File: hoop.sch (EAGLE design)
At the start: 33 parts, among them U1 PIC32MM0064GPL020-I/ML, U2 SGM2200

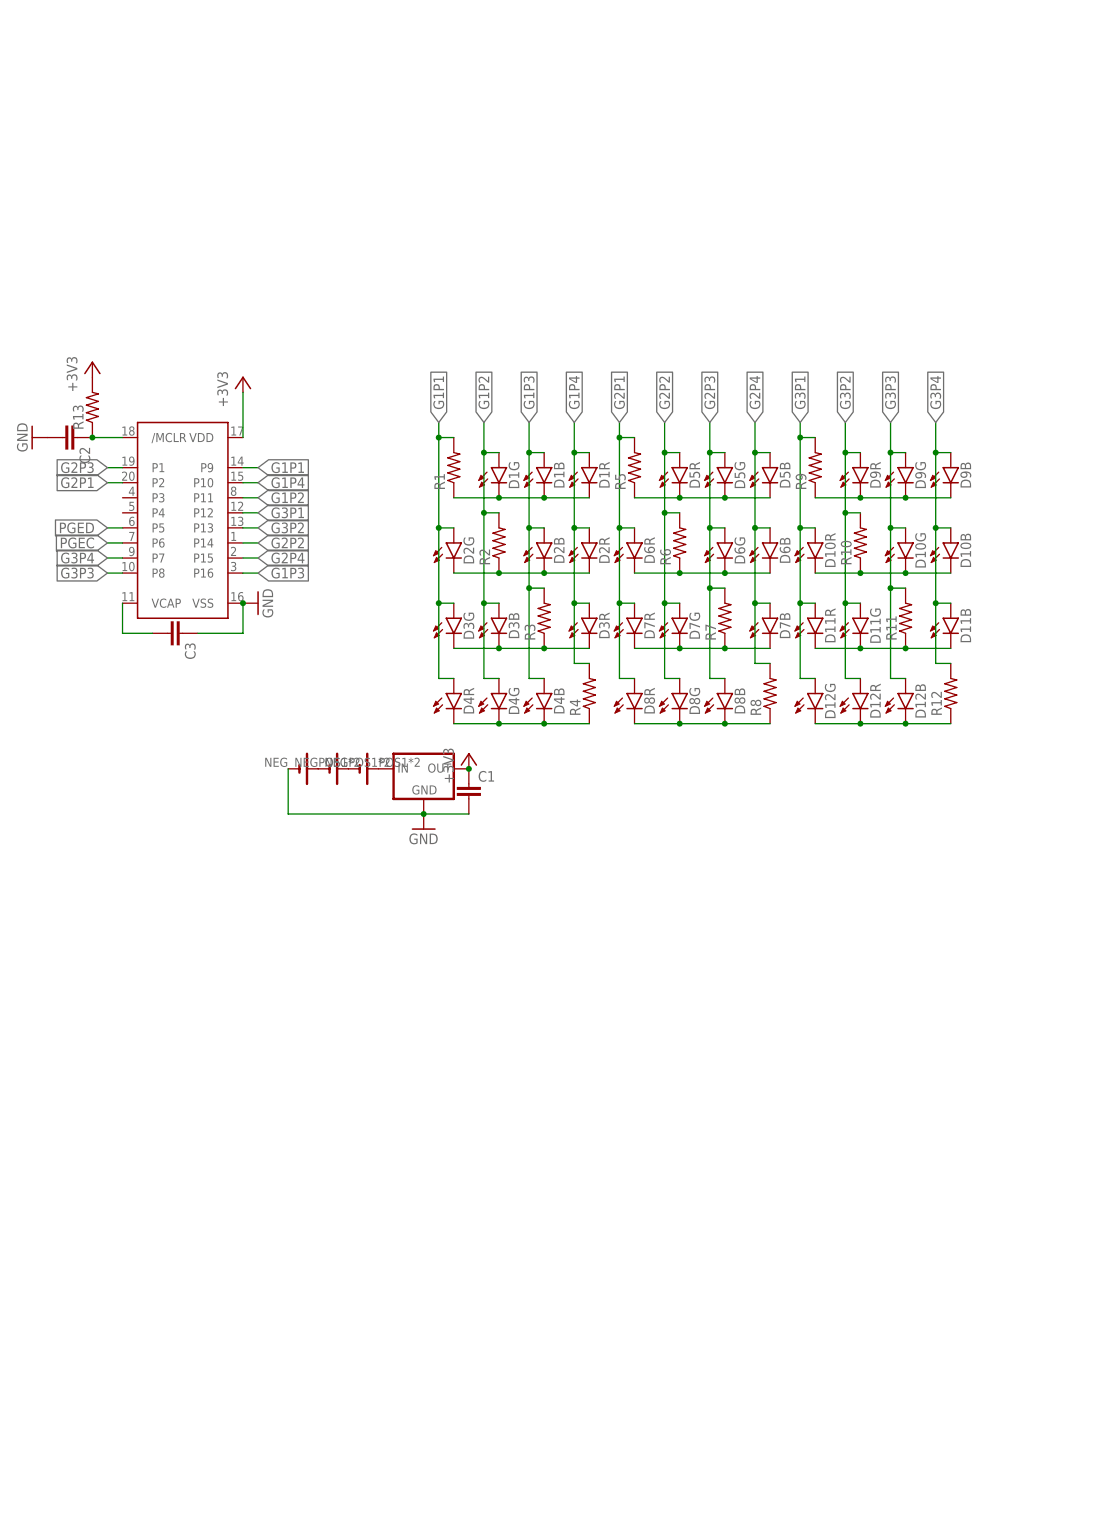
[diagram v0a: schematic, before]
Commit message: Cleaning up pcb files
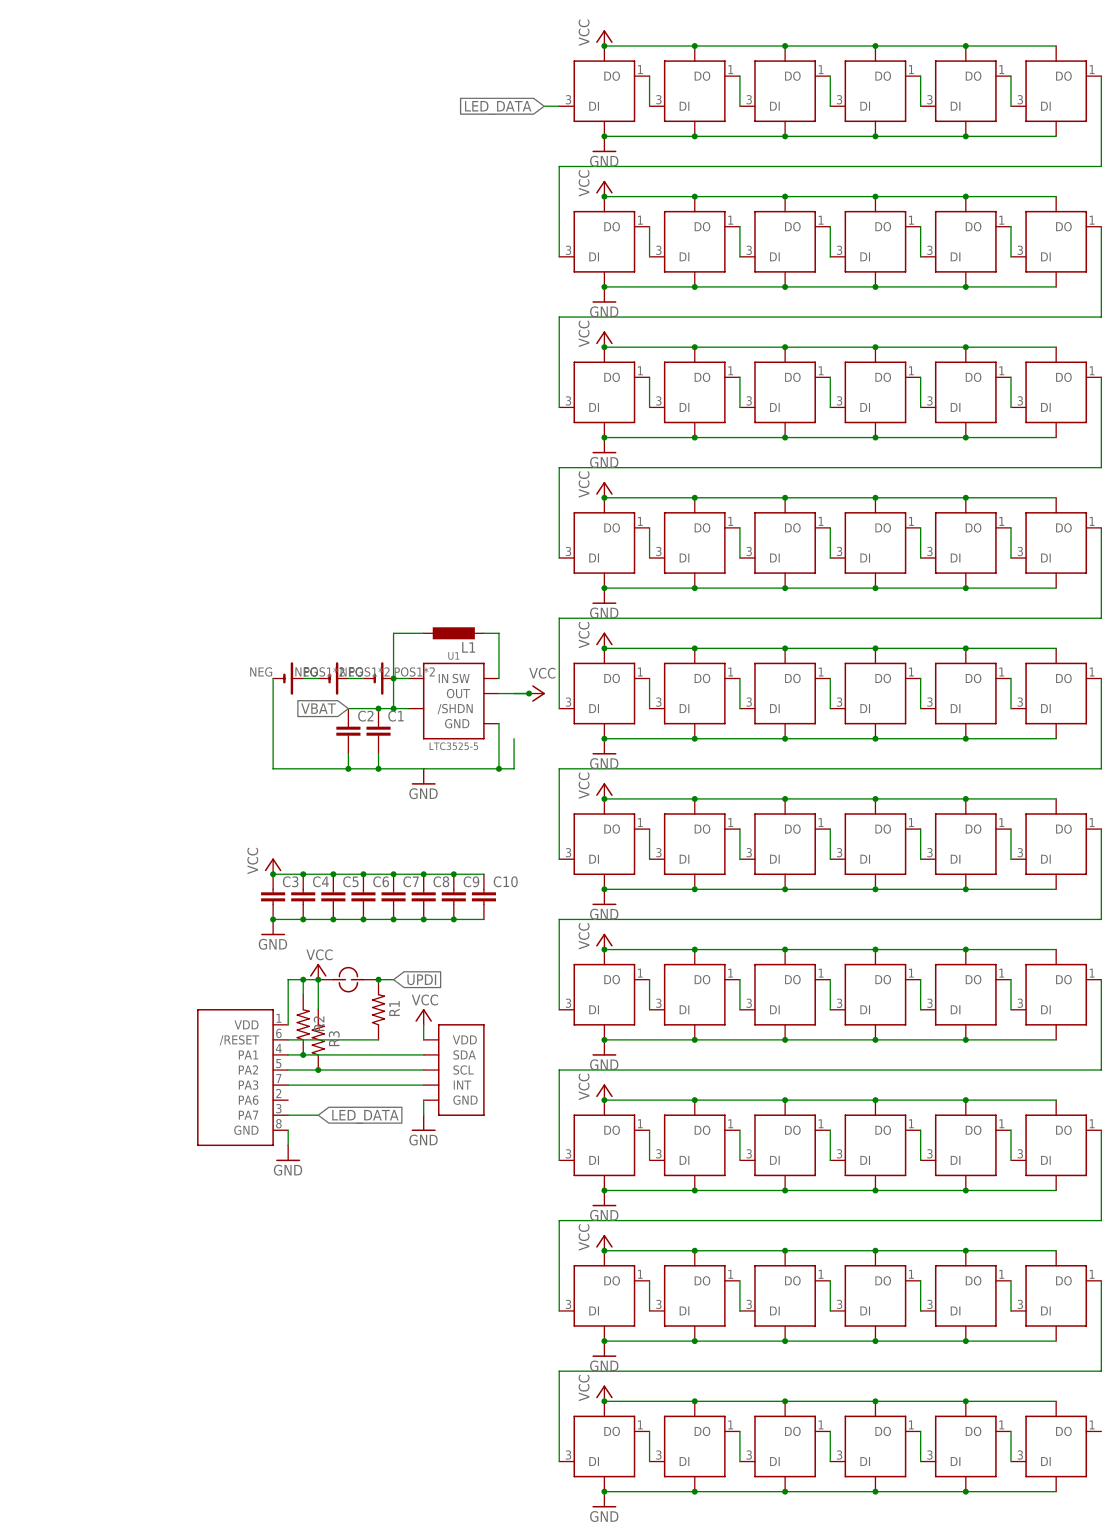
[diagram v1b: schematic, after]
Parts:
- removed R10, R11, R12, R4, R5, R6, R7, R8, R9: (no value), rcl:R-US_R0805
- removed R13: (no value), rcl:R-US_R0402
- added C10, C4, C5, C6, C7, C8, C9: (no value), rcl:C-EUC0805
- added D13, D14, D15, D16, D17, D18, D19, D20, D21, D22, D23, D24, D25, D26, D27, D28, D29, D30, D31, D32, D33, D34, D35, D36, D37, D38, D39, D40, D41, D42, D43, D44, D45, D46, D47, D48, D49, D50, D51, D52, D53, D54, D55, D56, D57, D58, D59, D60: SMD-LX0707RGB-TR, earring:SMD-LX0707RGB-TR
- added J1: JMP, earring:JMP
- added L1: (no value), rcl:L-EUL3216C
- added U3: ATTINY202, earring:ATTINY202
- C1, C2, C3: device rcl:C-EUC0402 -> rcl:C-EUC0805
- D1, D10, D11, D12, D2, D3, D4, D5, D6, D7, D8, D9: value FM-Z2727RGBA-SH -> SMD-LX0707RGB-TR; device earring:FM-Z2727RGBA-SH -> earring:SMD-LX0707RGB-TR
- U1: value PIC32MM0064GPL020-I/ML -> LTC3525; device earring:PIC32MM0064GPL020-I/ML -> earring:LTC3525
- U2: value SGM2200 -> MXC6255XU; device earring:SGM2200 -> earring:MXC6255XU
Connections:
- removed net +3V3: C1.1, R13.2, U1.VDD, U2.OUT
- removed net /MCLR: C2.1, R13.1, U1./MCLR
- removed net G1P1: D2G.A, D3G.A, D4R.A, R1.2, U1.P9
- removed net G1P2: D1G.A, D3B.A, D4G.A, R2.2, U1.P11
- removed net G1P3: D1B.A, D2B.A, D4B.A, R3.2, U1.P16
- removed net G1P4: D1R.A, D2R.A, D3R.A, R4.2, U1.P10
- removed net G2P1: D6R.A, D7R.A, D8R.A, R5.2, U1.P2
- removed net G2P2: D5R.A, D7G.A, D8G.A, R6.2, U1.P14
- removed net G2P3: D5G.A, D6G.A, D8B.A, R7.2, U1.P1
- removed net G2P4: D5B.A, D6B.A, D7B.A, R8.2, U1.P15
- removed net G3P1: D10R.A, D11R.A, D12G.A, R9.2, U1.P12
- removed net G3P2: D11G.A, D12R.A, D9R.A, R10.2, U1.P13
- removed net G3P3: D10G.A, D12B.A, D9G.A, R11.2, U1.P8
- removed net G3P4: D10B.A, D11B.A, D9B.A, R12.2, U1.P7
- removed net N$27: B3.+, U2.IN
- removed net PGEC: U1.P6
- removed net PGED: U1.P5
- new net LED_DATA: D1.DI, U3.PA7
- new net N$13: D15.DO, D16.DI
- new net N$14: D16.DO, D17.DI
- new net N$15: D17.DO, D18.DI
- new net N$16: D19.DO, D20.DI
- new net N$20: D23.DO, D24.DI
- new net N$21: D25.DO, D26.DI
- new net N$22: D26.DO, D27.DI
- new net N$23: D27.DO, D28.DI
- new net N$24: D28.DO, D29.DI
- new net N$28: D29.DO, D30.DI
- new net N$29: D31.DO, D32.DI
- new net N$30: D32.DO, D33.DI
- new net N$31: D33.DO, D34.DI
- new net N$32: D34.DO, D35.DI
- new net N$33: D35.DO, D36.DI
- new net N$34: D37.DO, D38.DI
- new net N$35: D38.DO, D39.DI
- new net N$36: D39.DO, D40.DI
- new net N$37: D40.DO, D41.DI
- new net N$38: D41.DO, D42.DI
- new net N$39: D43.DO, D44.DI
- new net N$40: D44.DO, D45.DI
- new net N$41: D45.DO, D46.DI
- new net N$42: D46.DO, D47.DI
- new net N$43: D47.DO, D48.DI
- new net N$44: D49.DO, D50.DI
- new net N$45: D50.DO, D51.DI
- new net N$46: D51.DO, D52.DI
- new net N$47: D52.DO, D53.DI
- new net N$48: D53.DO, D54.DI
- new net N$49: D55.DO, D56.DI
- new net N$5: D5.DO, D6.DI
- new net N$50: D56.DO, D57.DI
- new net N$51: D57.DO, D58.DI
- new net N$52: D58.DO, D59.DI
- new net N$53: D59.DO, D60.DI
- new net N$54: D6.DO, D7.DI
- new net N$55: D12.DO, D13.DI
- new net N$56: D18.DO, D19.DI
- new net N$57: D24.DO, D25.DI
- new net N$58: D30.DO, D31.DI
- new net N$59: D36.DO, D37.DI
- new net N$60: D42.DO, D43.DI
- new net N$61: D48.DO, D49.DI
- new net N$62: D54.DO, D55.DI
- new net N$64: L1.2, U1.SW
- new net N$66: U2.INT, U3.PA3
- new net N$69: R1.1, U3./RESET
- new net N$8: D10.DI, D9.DO
- new net SCL: R3.1, U2.SCL, U3.PA2
- new net SDA: R2.1, U2.SDA, U3.PA1
- new net UPDI: J1.P$2, R1.2
- new net VBAT: B3.+, C1.1, C2.1, L1.1, U1./SHDN, U1.IN
- new net VCC: C10.1, C3.1, C4.1, C5.1, C6.1, C7.1, C8.1, C9.1, D1.VDD, D10.VDD, D11.VDD, D12.VDD, D13.VDD, D14.VDD, D15.VDD, D16.VDD, D17.VDD, D18.VDD, D19.VDD, D2.VDD, D20.VDD, D21.VDD, D22.VDD, D23.VDD, D24.VDD, D25.VDD, D26.VDD, D27.VDD, D28.VDD, D29.VDD, D3.VDD, D30.VDD, D31.VDD, D32.VDD, D33.VDD, D34.VDD, D35.VDD, D36.VDD, D37.VDD, D38.VDD, D39.VDD, D4.VDD, D40.VDD, D41.VDD, D42.VDD, D43.VDD, D44.VDD, D45.VDD, D46.VDD, D47.VDD, D48.VDD, D49.VDD, D5.VDD, D50.VDD, D51.VDD, D52.VDD, D53.VDD, D54.VDD, D55.VDD, D56.VDD, D57.VDD, D58.VDD, D59.VDD, D6.VDD, D60.VDD, D7.VDD, D8.VDD, D9.VDD, J1.P$1, R2.2, R3.2, U1.OUT, U2.VDD, U3.VDD
- net GND: now also C10.2, C3.2, C4.2, C5.2, C6.2, C7.2, C8.2, C9.2, D1.GND, D10.GND, D11.GND, D12.GND, D13.GND, D14.GND, D15.GND, D16.GND, D17.GND, D18.GND, D19.GND, D2.GND, D20.GND, D21.GND, D22.GND, D23.GND, D24.GND, D25.GND, D26.GND, D27.GND, D28.GND, D29.GND, D3.GND, D30.GND, D31.GND, D32.GND, D33.GND, D34.GND, D35.GND, D36.GND, D37.GND, D38.GND, D39.GND, D4.GND, D40.GND, D41.GND, D42.GND, D43.GND, D44.GND, D45.GND, D46.GND, D47.GND, D48.GND, D49.GND, D5.GND, D50.GND, D51.GND, D52.GND, D53.GND, D54.GND, D55.GND, D56.GND, D57.GND, D58.GND, D59.GND, D6.GND, D60.GND, D7.GND, D8.GND, D9.GND, U1.GND, U3.GND; no longer C3.1, U1.VSS
- net N$1: now also D1.DO, D2.DI; no longer D1B.C, D1G.C, D1R.C, R1.1
- net N$10: now also D11.DO, D12.DI; no longer D6B.C, D6G.C, D6R.C, R6.1
- net N$11: now also D13.DO, D14.DI; no longer D7B.C, D7G.C, D7R.C, R7.1
- net N$12: now also D14.DO, D15.DI; no longer D8B.C, D8G.C, D8R.C, R8.1
- net N$17: now also D20.DO, D21.DI; no longer D9B.C, D9G.C, D9R.C, R9.1
- net N$18: now also D21.DO, D22.DI; no longer D10B.C, D10G.C, D10R.C, R10.1
- net N$19: now also D22.DO, D23.DI; no longer D11B.C, D11G.C, D11R.C, R11.1
- net N$2: now also D2.DO, D3.DI; no longer C3.2, U1.VCAP
- net N$3: now also D3.DO, D4.DI; no longer D2B.C, D2G.C, D2R.C, R2.1
- net N$4: now also D4.DO, D5.DI; no longer D4B.C, D4G.C, D4R.C, R4.1
- net N$6: now also D7.DO, D8.DI; no longer D3B.C, D3G.C, D3R.C, R3.1
- net N$7: now also D8.DO, D9.DI; no longer D12B.C, D12G.C, D12R.C, R12.1
- net N$9: now also D10.DO, D11.DI; no longer D5B.C, D5G.C, D5R.C, R5.1
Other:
- moved on the sheet: C1, C2, C3, R1, R2, R3
